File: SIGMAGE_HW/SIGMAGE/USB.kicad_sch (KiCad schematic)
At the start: 46 parts, among them J1 UJ31CHG2SMTTR, J3 TSW10607GS, J6 TSW10607GS, U13 ESDR0502NMUTBG, U14 93LC56-I/SN, U9 FT2232HLTRAY

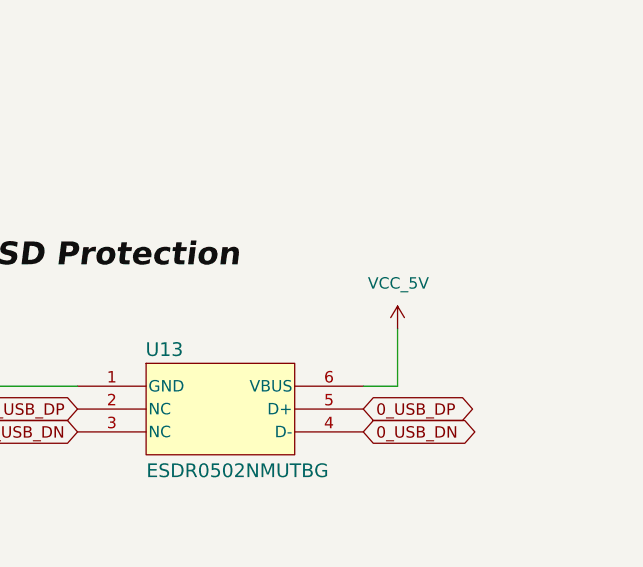
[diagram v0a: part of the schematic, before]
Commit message: before load switch and redoin power
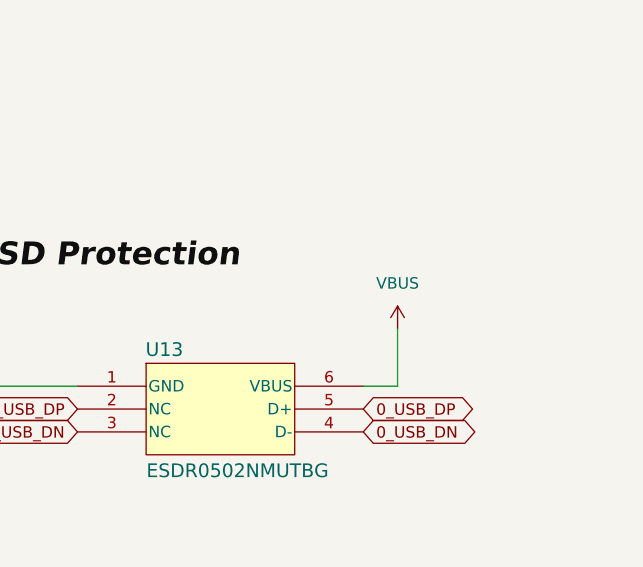
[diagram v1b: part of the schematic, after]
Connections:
- net VBUS: now also U13.6 (VBUS)
- net VCC_5V: no longer U13.6 (VBUS)
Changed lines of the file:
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@@
-	)
-	(symbol
-		(lib_id "power:+5V")
-		(at 367.03 209.55 0)
-		(unit 1)
-		(body_style 1)
-		(exclude_from_sim no)
-		(in_bom yes)
-		(on_board yes)
-		(in_pos_files yes)
-		(dnp no)
-		(property "Reference" "#PWR089"
-			(at 367.03 213.36 0)
-			(hide yes)
-			(show_name no)
-			(do_not_autoplace no)
-			(effects
-				(font
-					(size 1.27 1.27)
-				)
-			)
-		)
-		(property "Value" "VCC_5V"
-			(at 363.728 204.47 0)
-			(show_name no)
-			(do_not_autoplace no)
-			(effects
-				(font
-					(size 1.27 1.27)
-				)
-				(justify left)
-			)
-		)
-		(property "Footprint" ""
-			(at 367.03 209.55 0)
-			(hide yes)
-			(show_name no)
-			(do_not_autoplace no)
-			(effects
-				(font
-					(size 1.27 1.27)
-				)
-			)
-		)
-		(property "Datasheet" ""
-			(at 367.03 209.55 0)
-			(hide yes)
-			(show_name no)
-			(do_not_autoplace no)
-			(effects
-				(font
-					(size 1.27 1.27)
-				)
-			)
-		)
-		(property "Description" "Power symbol creates a global label with name \"+5V\""
-			(at 367.03 209.55 0)
-			(hide yes)
-			(show_name no)
-			(do_not_autoplace no)
-			(effects
-				(font
-					(size 1.27 1.27)
-				)
-			)
-		)
-		(pin "1"
-		)
-		(instances
-			(project "SIGMAGE"
-				(path "/6fbe3371-b6a3-4e28-aef4-4e5865f4674e/ccd460ba-3ae1-4da8-87e1-cc701b1f693c"
-					(reference "#PWR089")
-					(unit 1)
-				)
-			)
-		)
 	)
 	(symbol
@@
 					(unit 1)
 				)
+			)
+		)
+	)
+	(symbol
+		(lib_id "power:+5V")
+		(at 367.03 209.55 0)
+		(unit 1)
+		(body_style 1)
+		(exclude_from_sim no)
+		(in_bom yes)
+		(on_board yes)
+		(in_pos_files yes)
+		(dnp no)
+		(fields_autoplaced yes)
+		(property "Reference" "#PWR089"
+			(at 367.03 213.36 0)
+			(hide yes)
+			(show_name no)
+			(do_not_autoplace no)
+			(effects
+				(font
+					(size 1.27 1.27)
+				)
+			)
+		)
+		(property "Value" "VBUS"
+			(at 367.03 204.47 0)
+			(show_name no)
+			(do_not_autoplace no)
+			(effects
+				(font
+					(size 1.27 1.27)
+				)
+			)
+		)
+		(property "Footprint" ""
+			(at 367.03 209.55 0)
+			(hide yes)
+			(show_name no)
+			(do_not_autoplace no)
+			(effects
+				(font
+					(size 1.27 1.27)
+				)
+			)
+		)
+		(property "Datasheet" ""
+			(at 367.03 209.55 0)
+			(hide yes)
+			(show_name no)
+			(do_not_autoplace no)
+			(effects
+				(font
+					(size 1.27 1.27)
+				)
+			)
+		)
+		(property "Description" "Power symbol creates a global label with name \"+5V\""
+			(at 367.03 209.55 0)
+			(hide yes)
+			(show_name no)
+			(do_not_autoplace no)
+			(effects
+				(font
+					(size 1.27 1.27)
+				)
+			)
+		)
+		(pin "1"
+		)
+		(instances
+			(project "SIGMAGE"
+				(path "/6fbe3371-b6a3-4e28-aef4-4e5865f4674e/ccd460ba-3ae1-4da8-87e1-cc701b1f693c"
+					(reference "#PWR089")
+					(unit 1)
+				)
